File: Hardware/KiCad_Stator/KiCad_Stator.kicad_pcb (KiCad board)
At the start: 4 copper layers, 28 x 28 mm, 7 parts

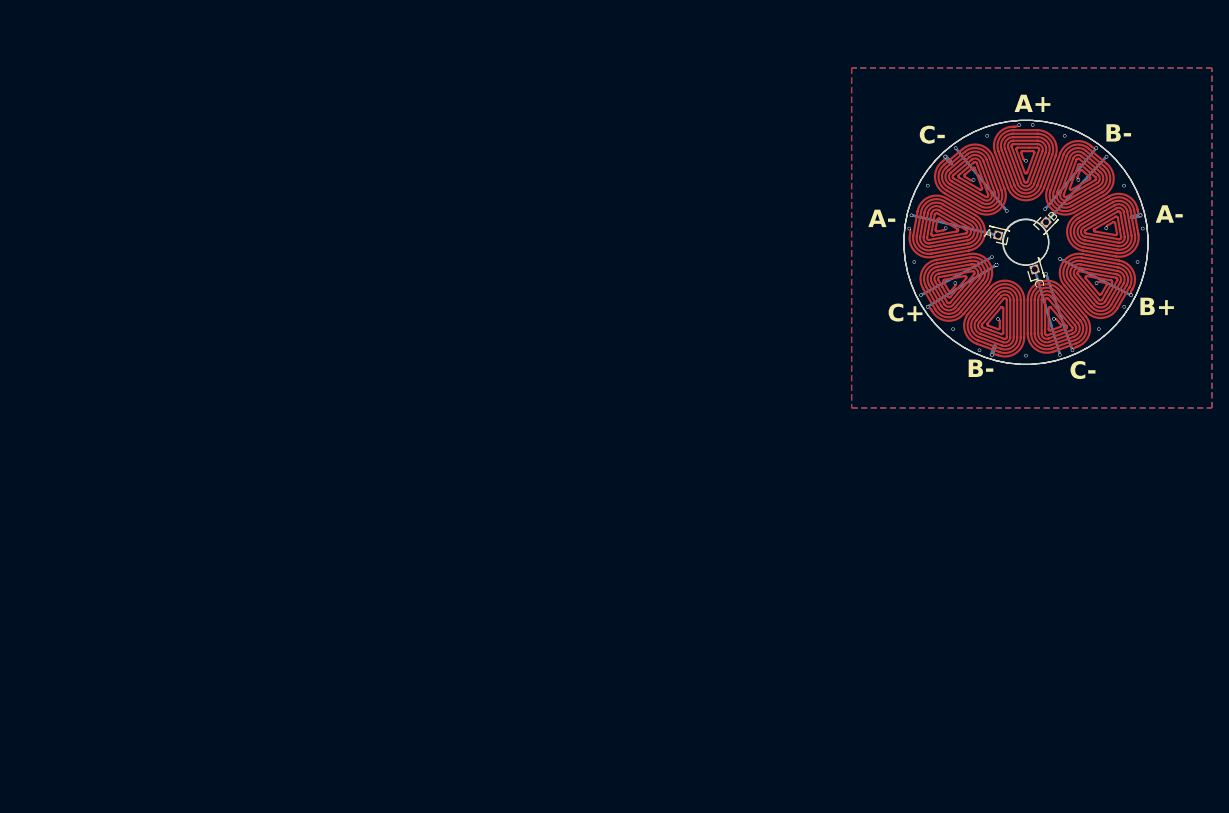
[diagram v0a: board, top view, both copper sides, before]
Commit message: feat:intro six layer
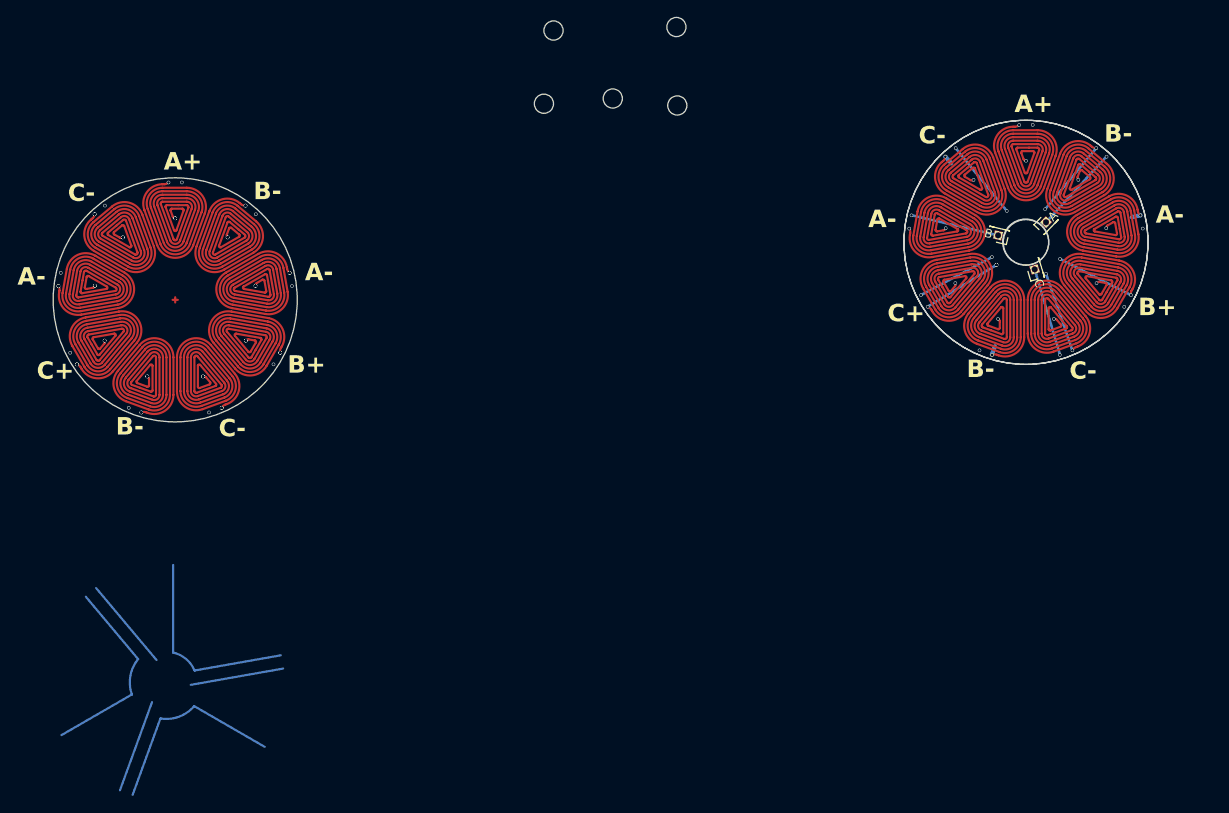
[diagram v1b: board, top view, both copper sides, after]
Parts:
- added H2: MountingHole, MountingHole:MountingHole_2.2mm_M2, F.Cu at (117.9, 49.3)
- added H3: MountingHole, MountingHole:MountingHole_2.2mm_M2, F.Cu at (103.8, 49.7)
- added H4: MountingHole, MountingHole:MountingHole_2.2mm_M2, F.Cu at (110.6, 57.5)
- added H5: MountingHole, MountingHole:MountingHole_2.2mm_M2, F.Cu at (102.7, 58.1)
- added H6: MountingHole, MountingHole:MountingHole_2.2mm_M2, F.Cu at (118.0, 58.3)
- A1: value B -> A
- B1: value A -> B
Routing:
- net GND: vias 9 -> 0
- net /C: vias 14 -> 29
- net /B: vias 9 -> 23
- net /A: vias 11 -> 26
- removed copper zone on B.Cu, net GND
- removed copper zone on F.Cu, net GND
- removed copper zone on In1.Cu, net GND
- removed copper zone on In2.Cu, net GND
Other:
- board size 28 x 28 mm -> 125.6 x 34.6 mm
- copper layers 4 -> 6
